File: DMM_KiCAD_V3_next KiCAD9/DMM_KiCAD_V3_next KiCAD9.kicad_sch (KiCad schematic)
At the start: 79 parts, among them J1 Conn_01x07_Pin, J10 ANALOG, J11 I_Input, J12 Conn_01x02_Pin, J13 DIGITAL1, J14 Barrel_Jack, J15 Barrel_Jack, J16 Conn_01x01_Socket, J17 Conn_01x01_Socket, J2 MicoSD, J3 Conn_01x07_Pin, J4 IR Connection, J5 POWER2, J6 POWER1, J7 Conn_01x02_Pin, J8 DIGITAL2, J9 Out to Screen, Q1 MMBT3904, Q2 SI2302 MOSFET, Q3 MMBT3904, Q4 MMBT3904, Q5 MMBT3904, Q6 BSS138, Q7 BSS138, SW1 SW_Push, SW2 SW_Push, SW3 SW_SPDT, SW4 SW_Push, U1 LM317_TO-220, U10 LM4040DBZ-2.5, U11 LM4040DBZ-5, U3 ADS1115IDGS, U7 MAX1683, U9 TPS613222ADBV

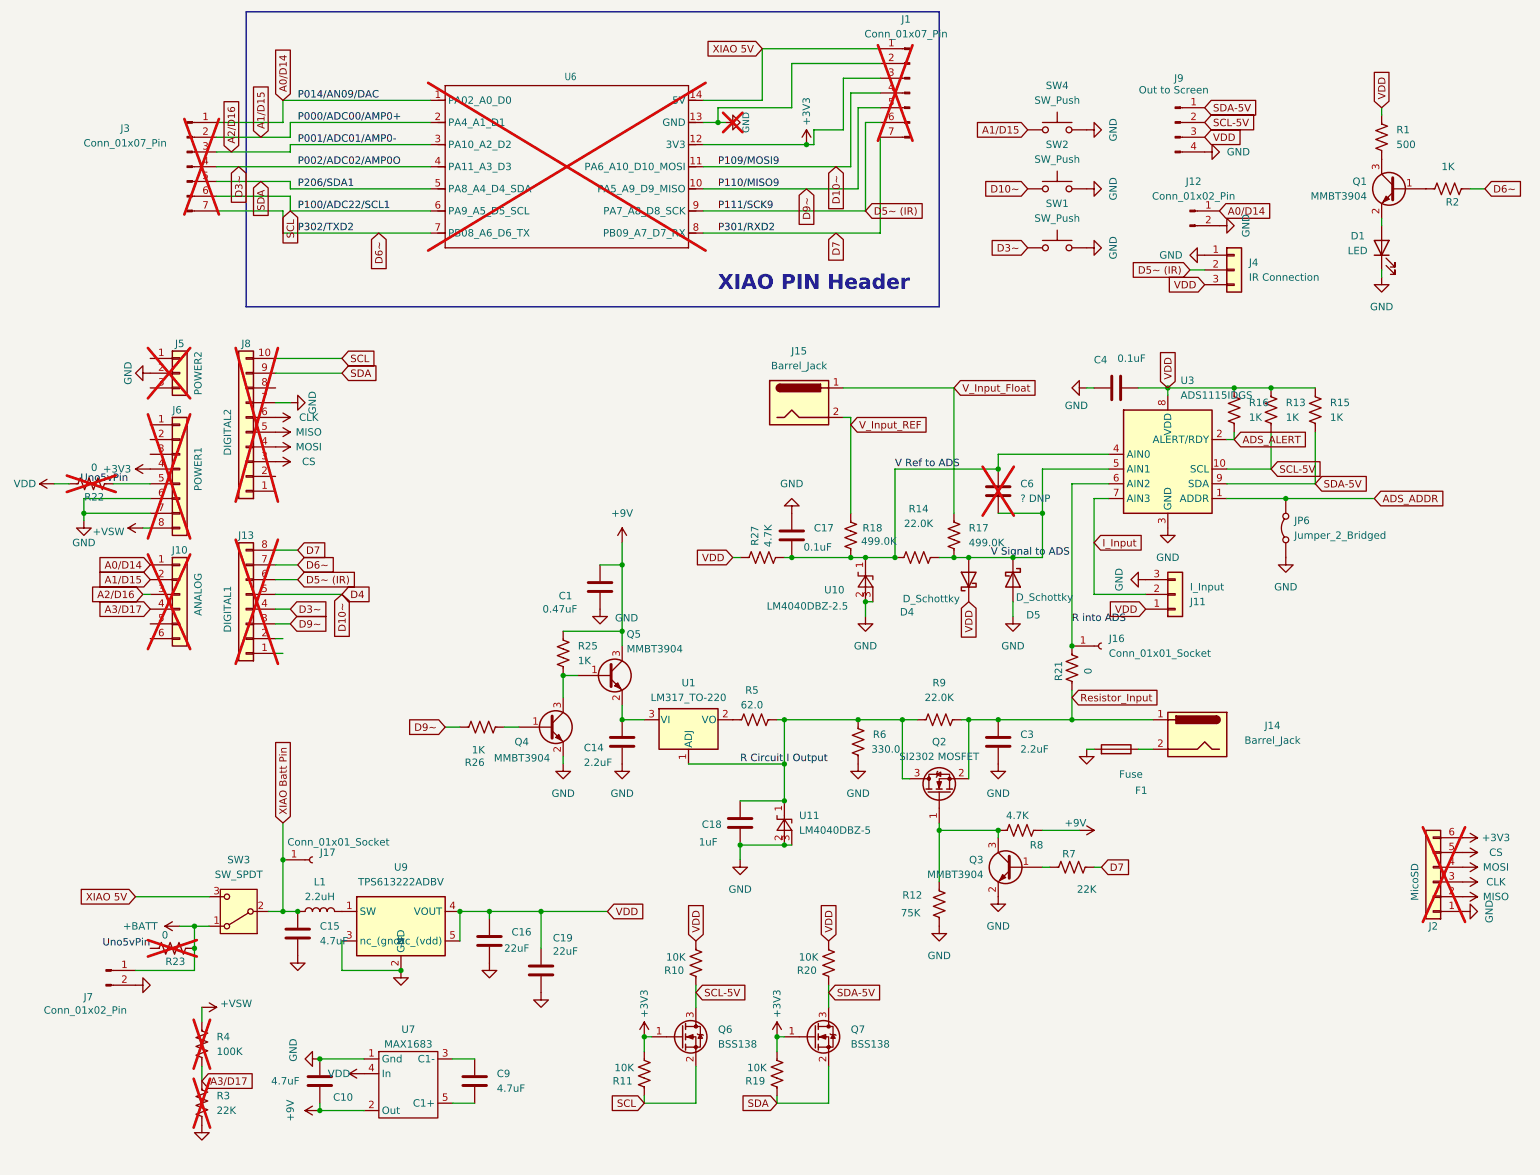
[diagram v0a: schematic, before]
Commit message: Mostly working on the next PCB
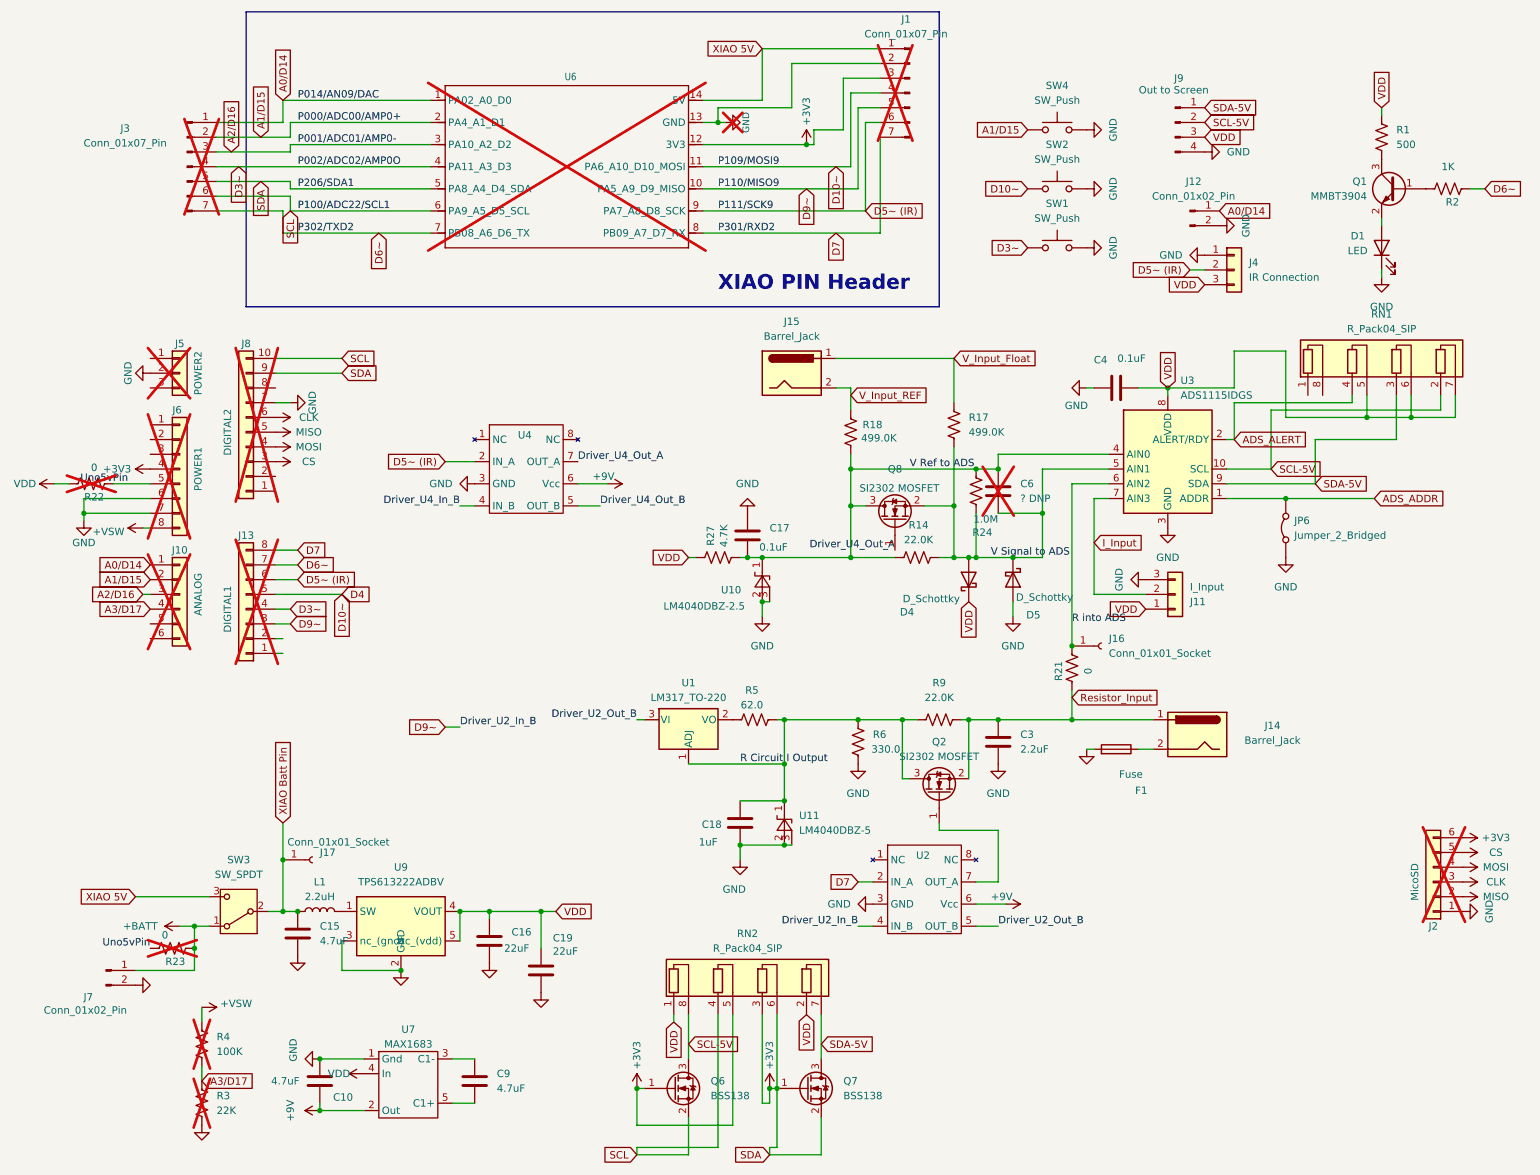
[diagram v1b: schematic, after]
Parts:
- removed C1: 0.47uF, Capacitor_SMD:C_0805_2012Metric_Pad1.18x1.45mm_HandSolder, symbol Device:C
- removed C14: 2.2uF, Capacitor_SMD:C_0805_2012Metric_Pad1.18x1.45mm_HandSolder, symbol Device:C
- removed Q3, Q4, Q5: MMBT3904, Package_TO_SOT_SMD:SOT-23, symbol Transistor_BJT:MMBT3904
- removed R10, R11, R19, R20: 10K, Resistor_SMD:R_0805_2012Metric_Pad1.20x1.40mm_HandSolder, symbol Device:R_US
- removed R12: 75K, Resistor_SMD:R_0805_2012Metric_Pad1.20x1.40mm_HandSolder, symbol Device:R_US
- removed R13, R15, R16, R25, R26: 1K, Resistor_SMD:R_0805_2012Metric_Pad1.20x1.40mm_HandSolder, symbol Device:R_US
- removed R7: 22K, Resistor_SMD:R_0805_2012Metric_Pad1.20x1.40mm_HandSolder, symbol Device:R_US
- removed R8: 4.7K, Resistor_SMD:R_0805_2012Metric_Pad1.20x1.40mm_HandSolder, symbol Device:R_US
- added Q8: SI2302 MOSFET, Package_TO_SOT_SMD:SOT-23, symbol Transistor_FET:DMG2302U
- added R24: 1.0M, Resistor_SMD:R_0805_2012Metric_Pad1.20x1.40mm_HandSolder, symbol Device:R_US
- added RN1, RN2: R_Pack04_SIP, Resistor_SMD:R_Array_Convex_4x1206, symbol Device:R_Pack04_SIP
- added U2, U4: ~, Package_SO:SOIC-8_3.9x4.9mm_P1.27mm, symbol CustomLibrary:IX4426_
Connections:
- net SDA is gone; now on net +3V3: J3.5 (Pin_5), J8.9 (Pin_9), Q7.2 (S), U6.5 (PA8_A4_D4_SDA)
- net +3V3: now also RN2.3 (R3.1), RN2.5 (R2.2), RN2.6 (R3.2)
- net +9V: now also U2.6 (Vcc), U4.6 (Vcc)
- net ADS_ALERT: now also RN1.4 (R2.1)
- net D5~ (IR): now also U4.2 (IN_A)
- net D7: now also U2.2 (IN_A)
- net D9~: now also U2.4 (IN_B)
- net GND: now also U2.3 (GND), U4.3 (GND)
- net SCL: now also RN2.4 (R2.1)
- net SCL-5V: now also RN1.2 (R4.1), RN2.8 (R1.2)
- net SDA-5V: now also RN1.3 (R3.1), RN2.7 (R4.2)
- net V Ref to ADS: now also Q8.3 (D), R24.2
- net V Signal to ADS: now also Q8.2 (S), R24.1
- net VDD: now also RN1.5 (R2.2), RN1.6 (R3.2), RN1.7 (R4.2), RN2.1 (R1.1), RN2.2 (R4.1)
- net at Q2.1 (G): now also U2.7 (OUT_A)
- net Driver_U2_Out_B: now reaches U1.3 (VI)
- net Driver_U2_Out_B: now also U2.5 (OUT_B)
- new net Driver_U4_In_B: U4.4 (IN_B)
- new net Driver_U4_Out_A: Q8.1 (G), U4.7 (OUT_A)
- new net Driver_U4_Out_B: U4.5 (OUT_B)
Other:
- moved on the sheet: C17, J15, Q6, Q7, R17, R18, R27, U10
